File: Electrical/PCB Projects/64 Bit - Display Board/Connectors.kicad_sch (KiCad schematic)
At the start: 16 parts, among them J1 Conn_01x03, J2 Conn_01x03, P1 610110249121, P2 610110249121, P3 610110249121

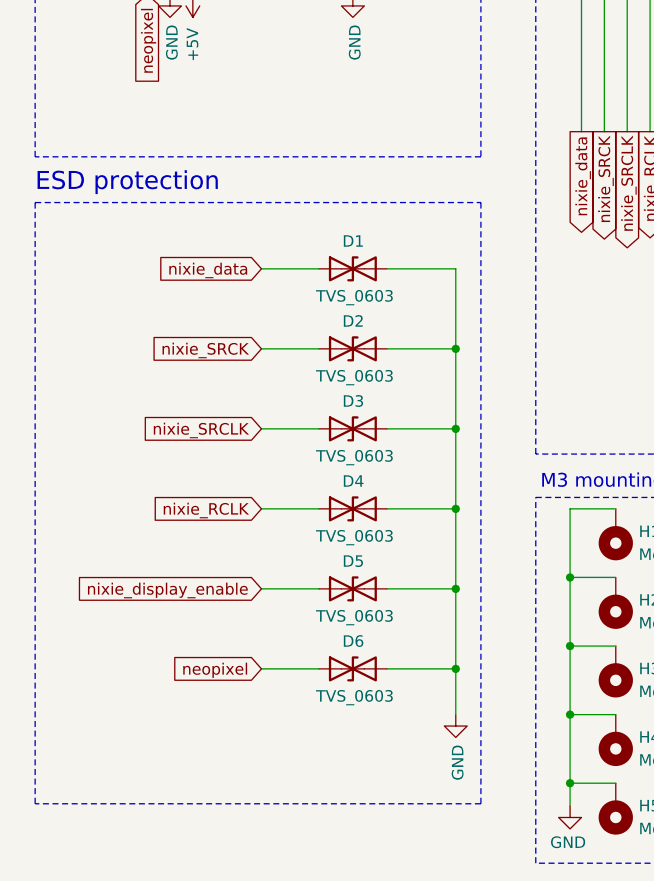
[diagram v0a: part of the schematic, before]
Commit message: slight changes
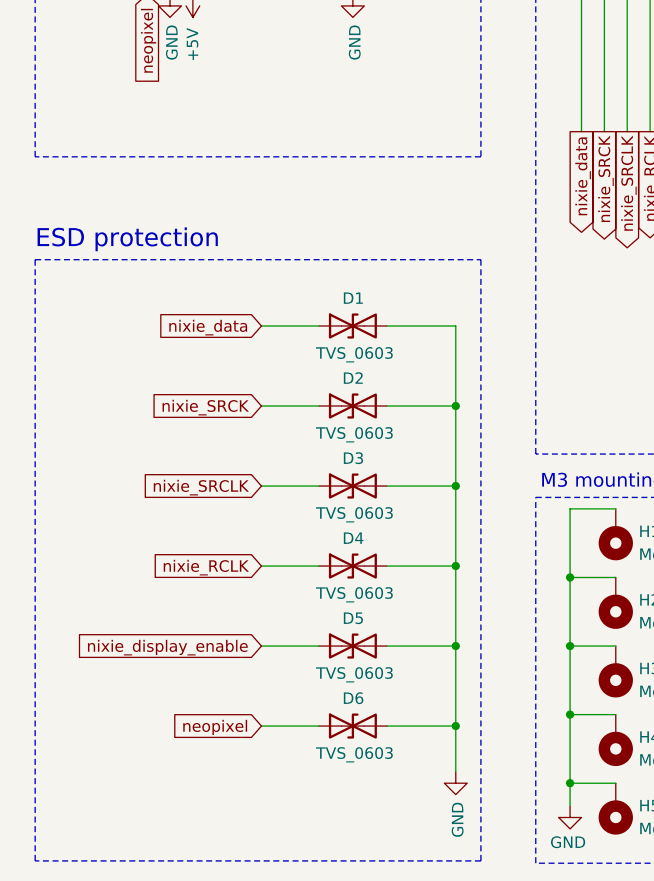
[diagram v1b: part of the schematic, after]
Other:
- moved on the sheet: D1, D2, D3, D4, D5, D6
